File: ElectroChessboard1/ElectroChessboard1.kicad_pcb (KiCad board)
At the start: 2 copper layers, 308.2 x 311.2 mm, 171 parts, among them IC1 A3213ELHLT-T, IC10 A3213ELHLT-T, IC11 A3213ELHLT-T, IC12 A3213ELHLT-T, IC13 A3213ELHLT-T, IC14 A3213ELHLT-T, IC15 A3213ELHLT-T, IC16 A3213ELHLT-T, IC17 A3213ELHLT-T, IC18 ADG708BRUZ-REEL7, IC19 A3213ELHLT-T, IC2 A3213ELHLT-T, IC20 A3213ELHLT-T, IC21 A3213ELHLT-T, IC22 A3213ELHLT-T, IC23 A3213ELHLT-T, IC24 A3213ELHLT-T, IC25 A3213ELHLT-T, IC26 A3213ELHLT-T, IC27 A3213ELHLT-T, IC28 A3213ELHLT-T, IC29 A3213ELHLT-T, IC3 A3213ELHLT-T, IC30 A3213ELHLT-T, IC31 A3213ELHLT-T, IC32 A3213ELHLT-T, IC33 A3213ELHLT-T, IC34 A3213ELHLT-T, IC35 ADG708BRUZ-REEL7, IC36 ADG708BRUZ-REEL7, IC37 A3213ELHLT-T, IC38 A3213ELHLT-T, IC39 A3213ELHLT-T, IC4 A3213ELHLT-T, IC40 A3213ELHLT-T, IC41 A3213ELHLT-T, IC42 A3213ELHLT-T, IC43 A3213ELHLT-T, IC44 A3213ELHLT-T, IC45 A3213ELHLT-T, IC46 A3213ELHLT-T, IC47 A3213ELHLT-T, IC48 A3213ELHLT-T, IC49 A3213ELHLT-T, IC5 A3213ELHLT-T, IC50 A3213ELHLT-T, IC51 A3213ELHLT-T, IC52 A3213ELHLT-T, IC53 ADG708BRUZ-REEL7, IC54 ADG708BRUZ-REEL7, IC55 A3213ELHLT-T, IC56 A3213ELHLT-T, IC57 A3213ELHLT-T, IC58 A3213ELHLT-T, IC59 A3213ELHLT-T, IC6 A3213ELHLT-T, IC60 A3213ELHLT-T, IC61 A3213ELHLT-T, IC62 A3213ELHLT-T, IC63 A3213ELHLT-T, IC64 A3213ELHLT-T, IC65 A3213ELHLT-T, IC66 A3213ELHLT-T, IC67 A3213ELHLT-T, IC68 A3213ELHLT-T, IC69 A3213ELHLT-T, IC7 A3213ELHLT-T, IC70 A3213ELHLT-T, IC71 ADG708BRUZ-REEL7, IC72 ADG708BRUZ-REEL7, IC73 CD74HC154M96, IC74 CD74HC154M96, IC75 DS1307Z+T&R, IC8 A3213ELHLT-T, IC9 ADG708BRUZ-REEL7, J1 USB_B, J3 Conn_01x04_Pin, J5 Conn_01x06, J6 Conn_01x06, U1 ATmega2560-16A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

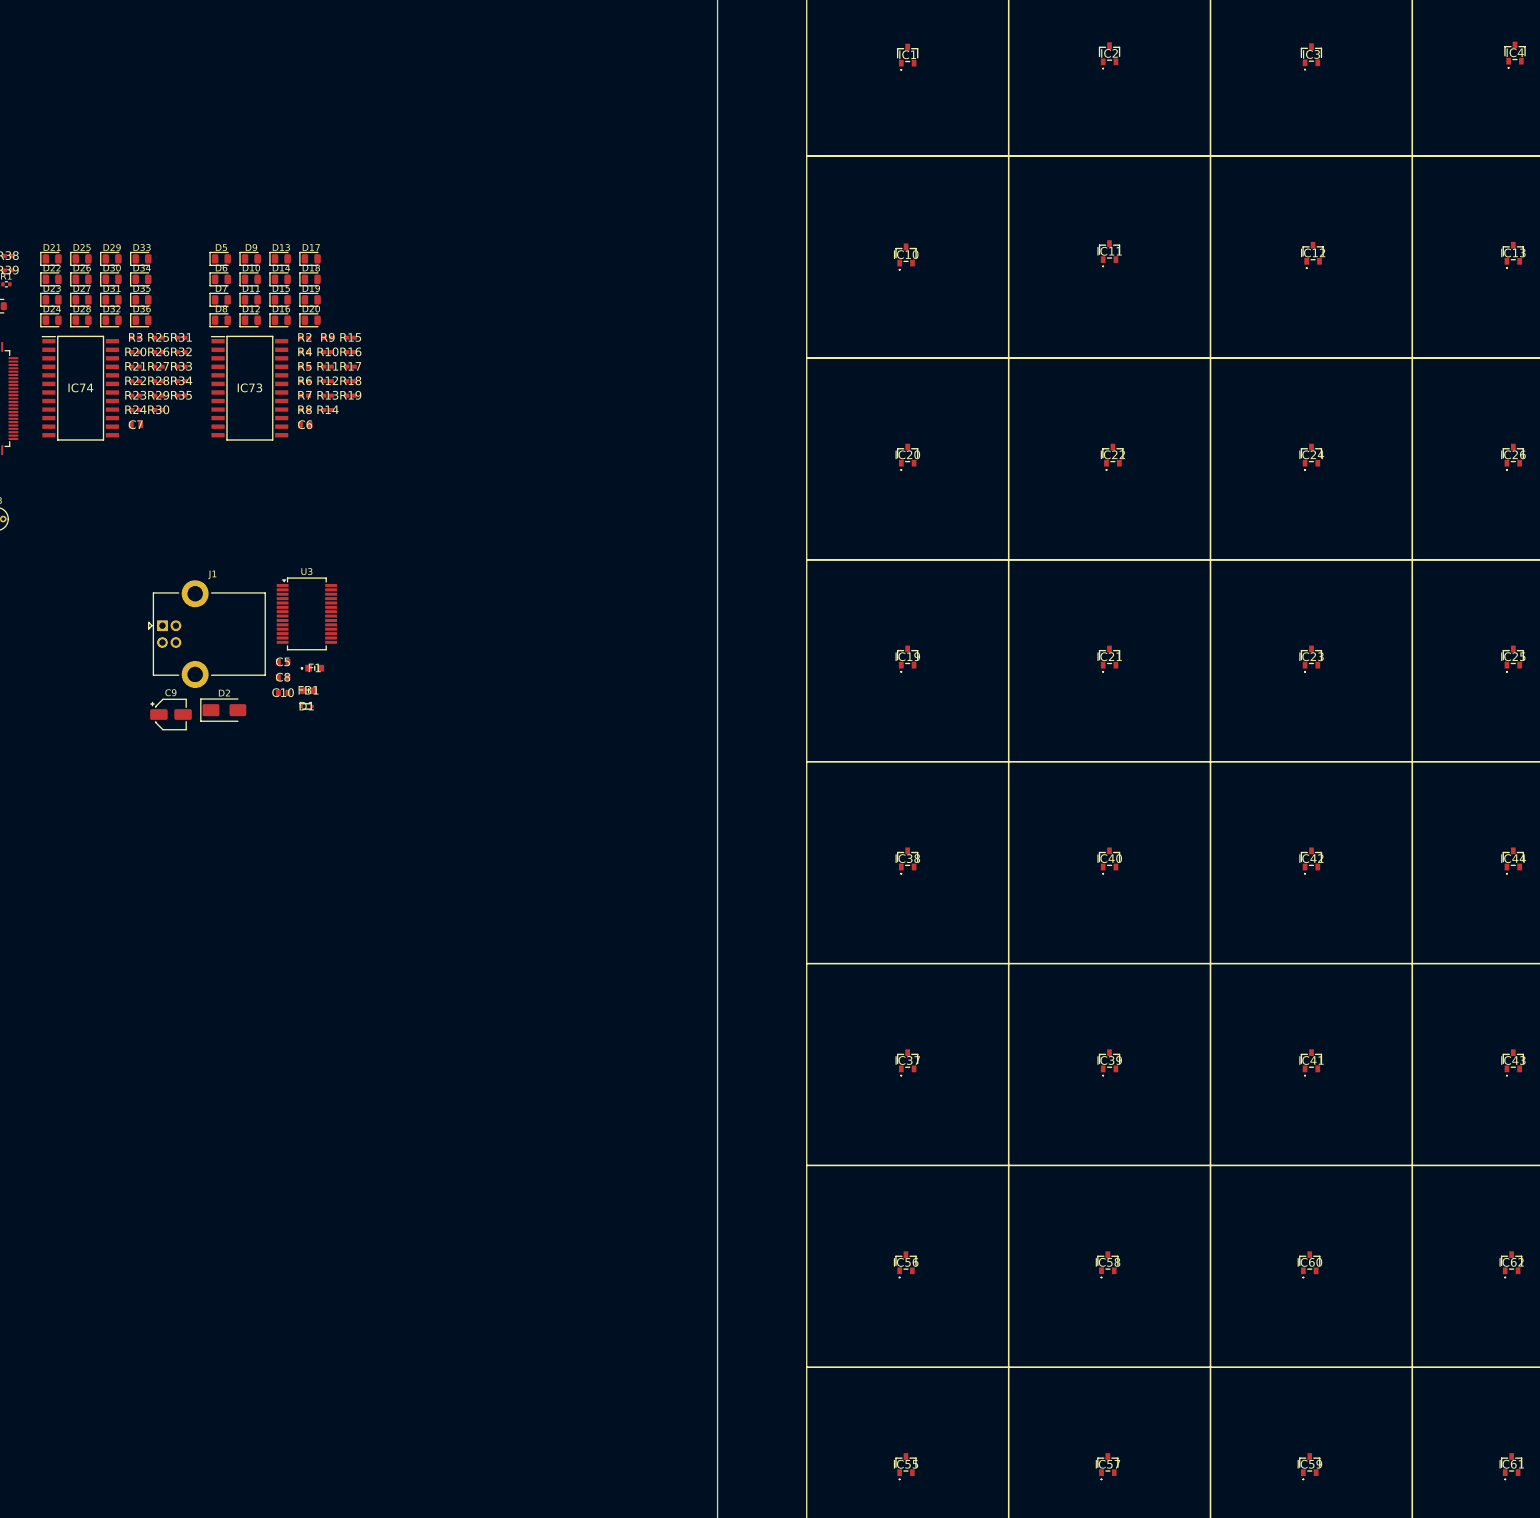
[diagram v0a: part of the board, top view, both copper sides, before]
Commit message: update
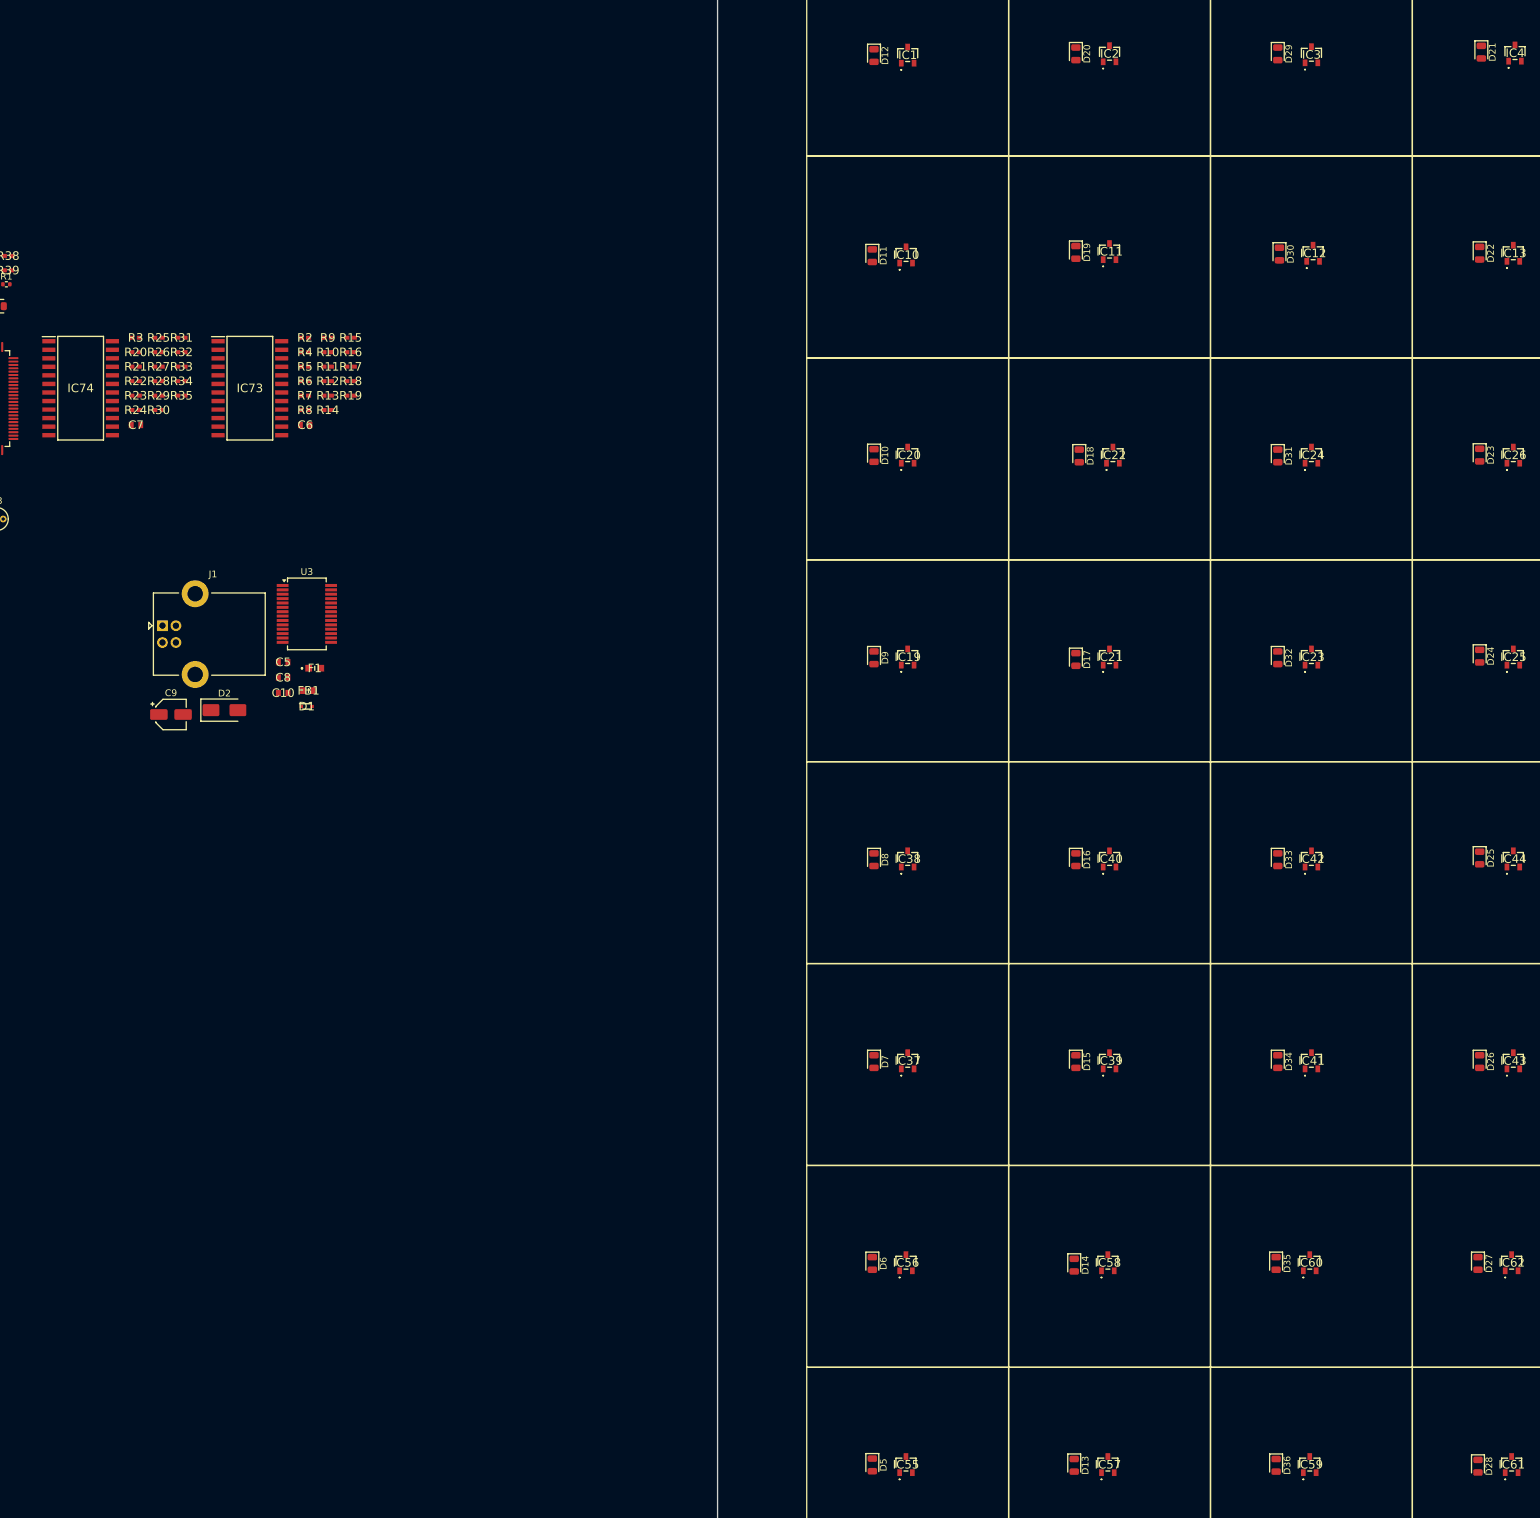
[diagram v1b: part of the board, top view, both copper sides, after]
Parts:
- moved D28 268.4 mm to (134.2, 254.9), turned to -90 degrees
- moved D27 252.1 mm to (134.2, 224.8), turned to -90 degrees
- moved D36 239.5 mm to (104.2, 254.8), turned to -90 degrees
- moved D26 238.0 mm to (134.5, 194.8), turned to -90 degrees
- moved D25 226.0 mm to (134.5, 164.6), turned to -90 degrees
- moved D35 221.2 mm to (104.2, 224.8), turned to -90 degrees
- moved D24 217.9 mm to (134.5, 134.6), turned to -90 degrees
- moved D21 214.6 mm to (134.8, 44.8), turned to -90 degrees
- moved D13 214.5 mm to (74.2, 254.8), turned to -90 degrees
- moved D23 213.4 mm to (134.5, 104.7), turned to -90 degrees
- moved D22 212.2 mm to (134.5, 74.7), turned to -90 degrees
- moved D34 204.9 mm to (104.5, 194.8), turned to -90 degrees
- moved D5 203.7 mm to (44.2, 254.8), turned to -90 degrees
- moved D33 190.9 mm to (104.5, 164.8), turned to -90 degrees
- moved D14 188.0 mm to (74.2, 225.1), turned to -90 degrees
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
